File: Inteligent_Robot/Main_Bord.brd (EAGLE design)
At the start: 132.1 x 101.6 mm, 83 parts, among them CN5 DF11-4DS-2C, CN6 DF11-4DS-2C, CN7 IL-G_ST_4, CN8 IL-G_ST_4, IC1 TWE-001L-IP, IC2 LTC2862A, IC5 A4988, IC7 A4988

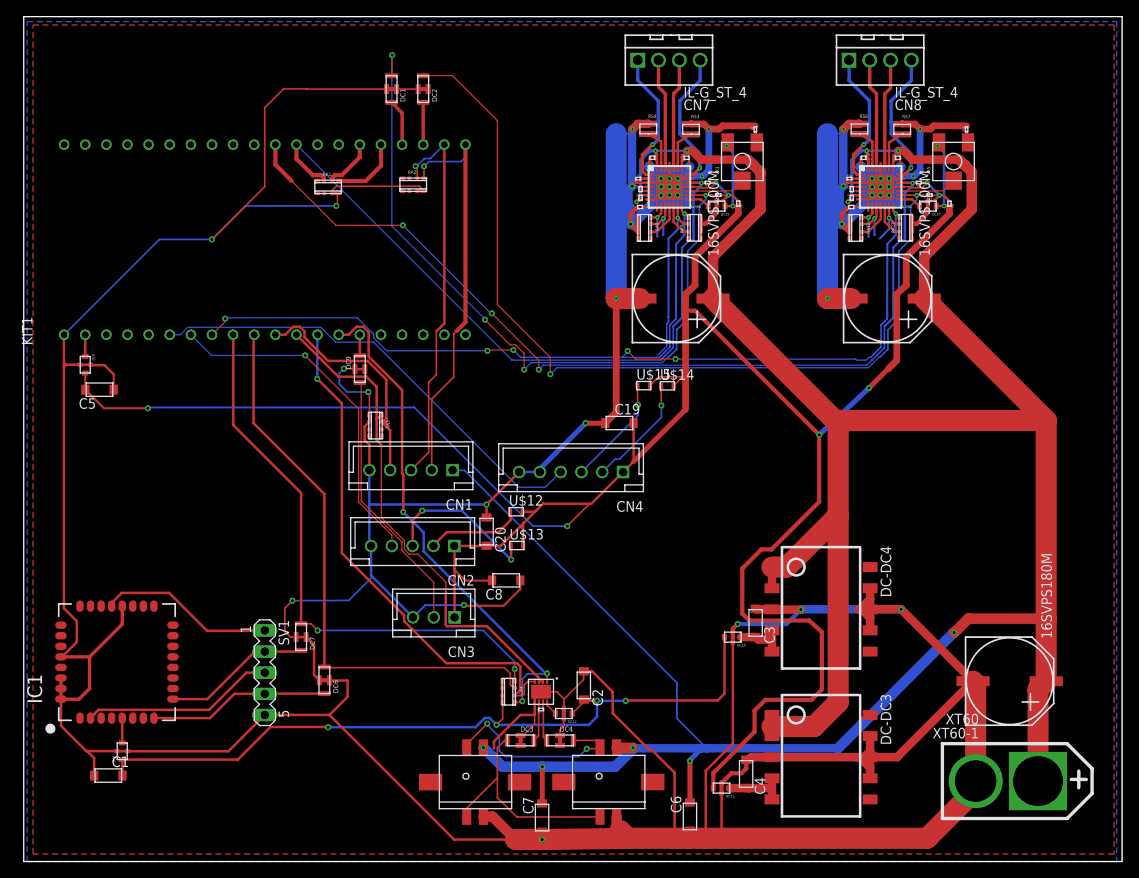
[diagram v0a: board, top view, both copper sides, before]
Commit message: Ver2
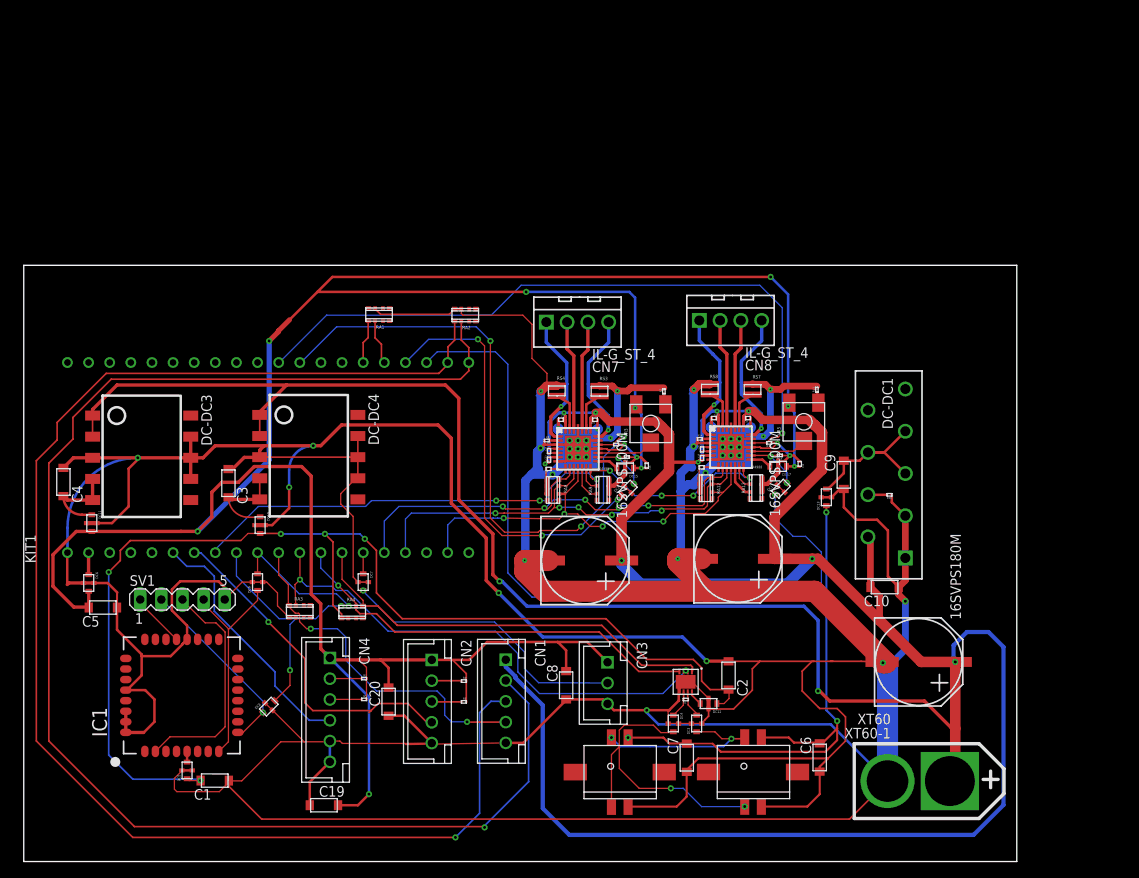
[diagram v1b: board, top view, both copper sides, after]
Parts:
- removed U$12, U$13, U$14, U$15: MCR03, ROHM:MCR03
- removed U$9: 16SVPS180M, OS-CON:SVCP_F8
- added C10, C9: GMR31, Murata:GMR31
- added DC-DC1: MPM01, SANKEN:MPM00_V
- added DC13: YFF21PC, TDK:YFF21PC
- added OS-CON1: 16SVPS180M, OS-CON:SVCP_F8
- added R10, R2, R5, R6, R9: MCR006, ROHM:MCR006
- DC1, DC2, DC3, DC4, DC6, DC7, DC9: value NFM3DPC223R1H3L -> YFF21PC; device Murata:NFM3DC -> TDK:YFF21PC
- moved C4 89.3 mm to (5.35, 43.9)
- moved DC-DC3 89.3 mm to (20.7, 53.6)
- moved DC11 82.2 mm to (8.77, 40.7), turned to 90 degrees
- moved DC1 66.0 mm to (91.6, 44.8), turned to 225 degrees
- moved C3 65.6 mm to (25.2, 43.8)
- moved DC-DC4 64.3 mm to (40.8, 53.7)
- moved DC10 58.4 mm to (29.0, 40.5), turned to 90 degrees
- moved C19 58.1 mm to (38.4, 6.77)
- moved DC2 52.7 mm to (73.2, 44.7), turned to 225 degrees
- moved DC8 46.7 mm to (30.1, 18.6), turned to 225 degrees
- moved CN4 40.7 mm to (37.4, 18.2), turned to 270 degrees
- moved C34 36.1 mm to (83.9, 53.3)
- moved C35 36.1 mm to (82.2, 48.8)
- moved C36 36.1 mm to (82.2, 49.9)
- moved C39 36.1 mm to (87.4, 53.3)
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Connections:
- new net +7.5V: C6.P$1, C7.P$1, CN5.P$3, CN6.P$3, DC13.P$2
- new net N$6: C9.P$1, DC-DC1.P$5, DC-DC1.P$6, DC-DC1.P$7, DC13.P$1
- new net N$9: DC-DC1.P$4, R10.P$1
- net +5V: now also DC6.P$1, R2.P$1, R5.P$1, R6.P$1, R9.P$1; no longer DC8.P$1, U$12.P$1, U$13.P$1, U$14.P$1, U$15.P$1
- net A*: now also DC4.P$1; no longer DC3.P$2
- net B*: now also DC3.P$2; no longer DC4.P$1
- net GND: now also C10.P$2, C9.P$2, DC-DC1.P$1, DC-DC1.P$3, DC1.GND1, DC1.GND2, DC13.GND1, DC13.GND2, DC2.GND1, DC2.GND2, DC3.GND1, DC3.GND2, DC4.GND1, DC4.GND2, DC6.GND1, DC6.GND2, DC7.GND1, DC7.GND2, DC9.GND1, DC9.GND2, OS-CON1.P$1, R10.P$2; no longer DC1.P$3, DC1.P$4, DC2.P$3, DC2.P$4, DC3.P$3, DC3.P$4, DC4.P$3, DC4.P$4, DC6.P$3, DC6.P$4, DC7.P$3, DC7.P$4, DC9.P$3, DC9.P$4, U$9.P$1
- net MOTOR_INT: now also RA3.P$1; no longer RA3.P$2
- net MS1: now also KIT1.P$16
- net MS2: now also KIT1.P$17
- net MS3: now also KIT1.P$19
- net M_TO_T-1: now also DC9.P$1; no longer DC6.P$2
- net M_TO_T-2: now also DC8.P$1; no longer DC7.P$2
- net N$1: now also RA2.P$3; no longer RA2.P$4
- net N$14: now also DC4.P$2; no longer DC3.P$1
- net N$15: now also DC3.P$1; no longer DC4.P$2
- net N$2: now also RA2.P$4; no longer RA2.P$3
- net N$3: now also DC6.P$2; no longer DC8.P$2
- net N$36: now also DC2.P$2; no longer DC1.P$1
- net N$37: now also DC1.P$2; no longer DC2.P$1
- net N$38: now also R9.P$2; no longer U$12.P$2
- net N$39: now also R6.P$2; no longer U$13.P$2
- net N$40: now also R2.P$2; no longer U$14.P$2
- net N$41: now also R5.P$2; no longer U$15.P$2
- net N$5: now also DC7.P$2; no longer DC9.P$1
- net N$7: now also RA1.P$3; no longer RA1.P$4
- net N$8: now also RA1.P$4; no longer RA1.P$3
- net PSD: now also DC7.P$1; no longer DC9.P$2
- net RT-T: now also DC8.P$2; no longer DC7.P$1
- net SEL_485: now also RA3.P$2; no longer RA3.P$1
- net STP1: now also DC2.P$1; no longer DC1.P$2
- net STP2: now also DC1.P$1; no longer DC2.P$2
- net TX-T: now also DC9.P$2; no longer DC6.P$1
- net VDD: now also C10.P$1, DC-DC1.P$2, OS-CON1.P$2+; no longer C6.P$1, C7.P$1, CN5.P$3, CN6.P$3, U$9.P$2+
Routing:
- net N$1: track 49.3 -> 174.1 mm
- net N$2: track 46.9 -> 169.9 mm
- net STP2: track 109.3 -> 7.29 mm
- net N$37: track 5.08 -> 89.5 mm, vias 0 -> 1
- net STP1: track 90.1 -> 7.15 mm, vias 4 -> 2
- net +7.5V: track 0.00 -> 65.4 mm, vias 0 -> 3
- net GND: track 862.9 -> 919.3 mm, vias 34 -> 30
- net M_TO_T-1: track 68.2 -> 16.2 mm, vias 0 -> 1
- net SLEEP1: track 129.0 -> 77.1 mm
- net MS1: track 9.17 -> 57.5 mm, vias 2 -> 5
- net N$36: track 5.61 -> 51.1 mm, vias 0 -> 3
- net +3.3V: track 95.8 -> 141.2 mm, vias 4 -> 5
- net MS2: track 10.6 -> 54.3 mm, vias 2 -> 5
- net MS3: track 8.81 -> 51.3 mm, vias 0 -> 4
- net M_TO_T-2: track 68.2 -> 29.2 mm
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- removed copper zone on layer 1, net GND
- removed copper zone on layer 16, net GND
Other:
- board size 132.1 x 101.6 mm -> 119.4 x 71.7 mm

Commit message: update
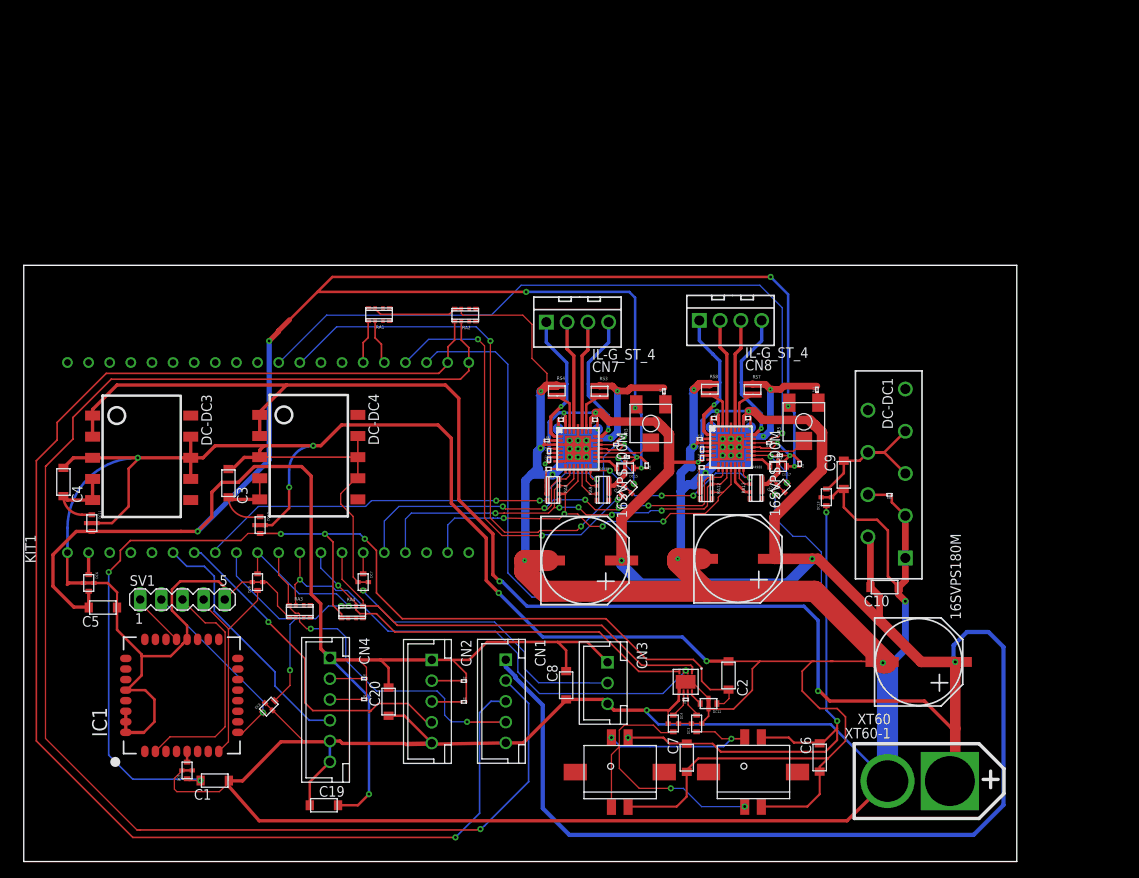
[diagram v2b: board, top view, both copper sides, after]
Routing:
- net GND: track 919.3 -> 921.7 mm
- net N$1: track 174.1 -> 175.1 mm
